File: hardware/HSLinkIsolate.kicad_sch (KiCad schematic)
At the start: 57 parts, among them J101 USB_B, J102 ISP, J103 IDC, Q101 AO3400A, SW101 BOOT, U101 HPM5301IEG1, U102 USBLC6-2SC6, U103 ISO7741, U104 ISO7741, U105 SN74LVC1G125DBV, U107 RT9193, Y101 24MHz

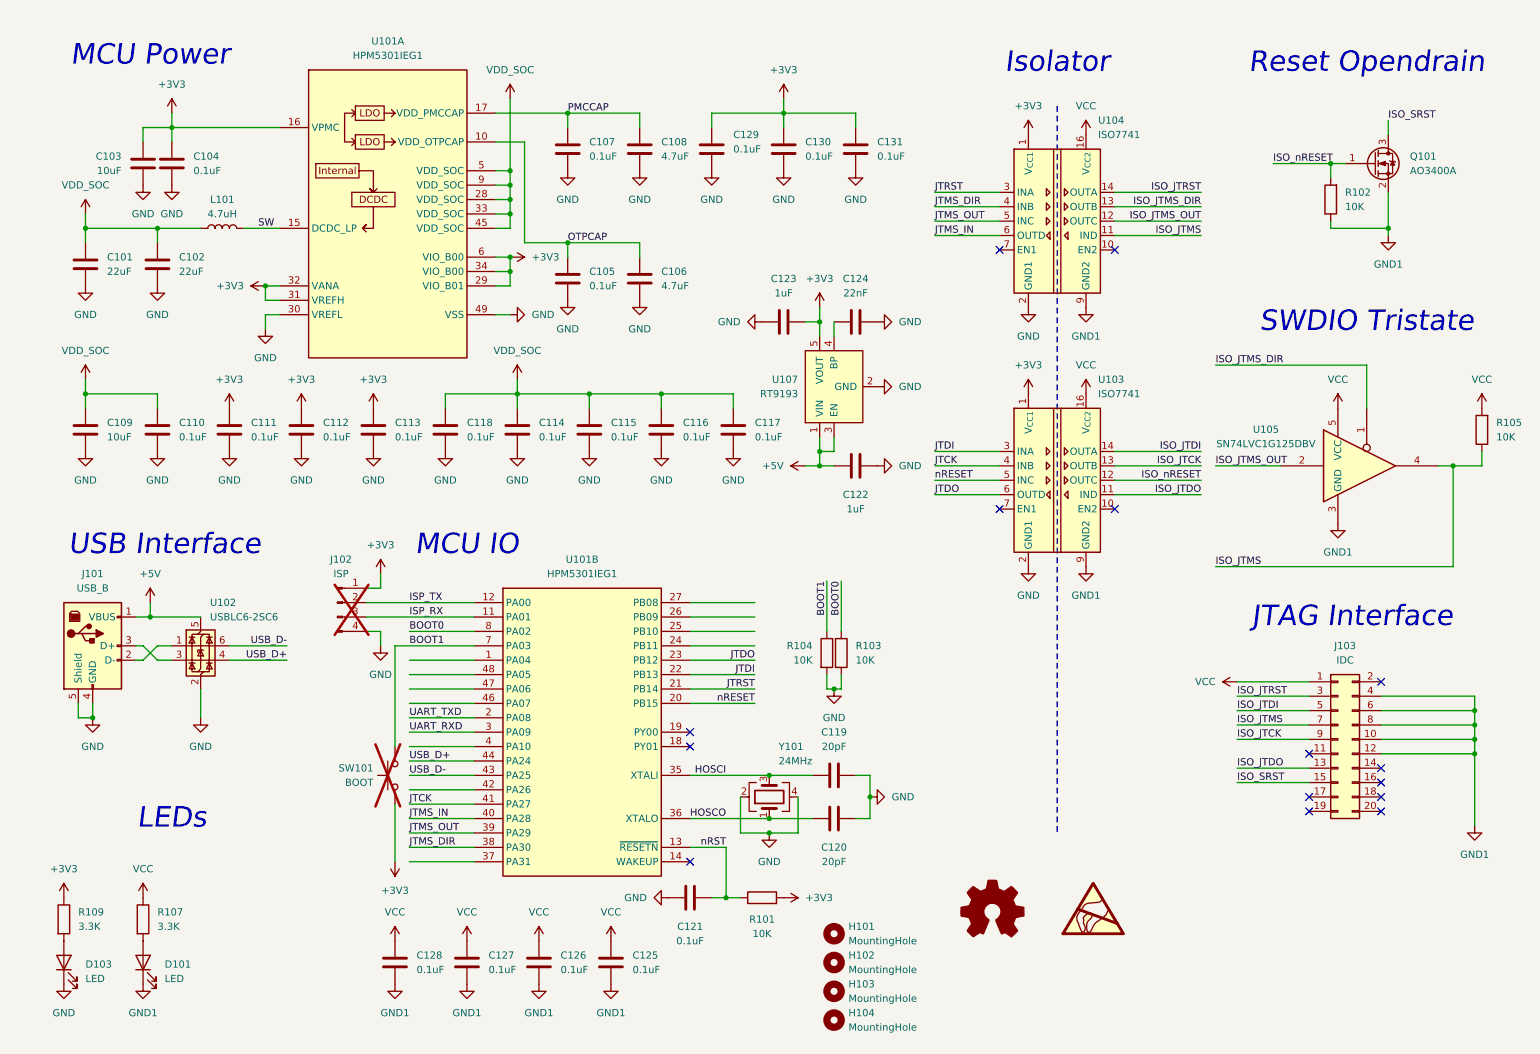
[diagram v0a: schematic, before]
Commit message: update hardware
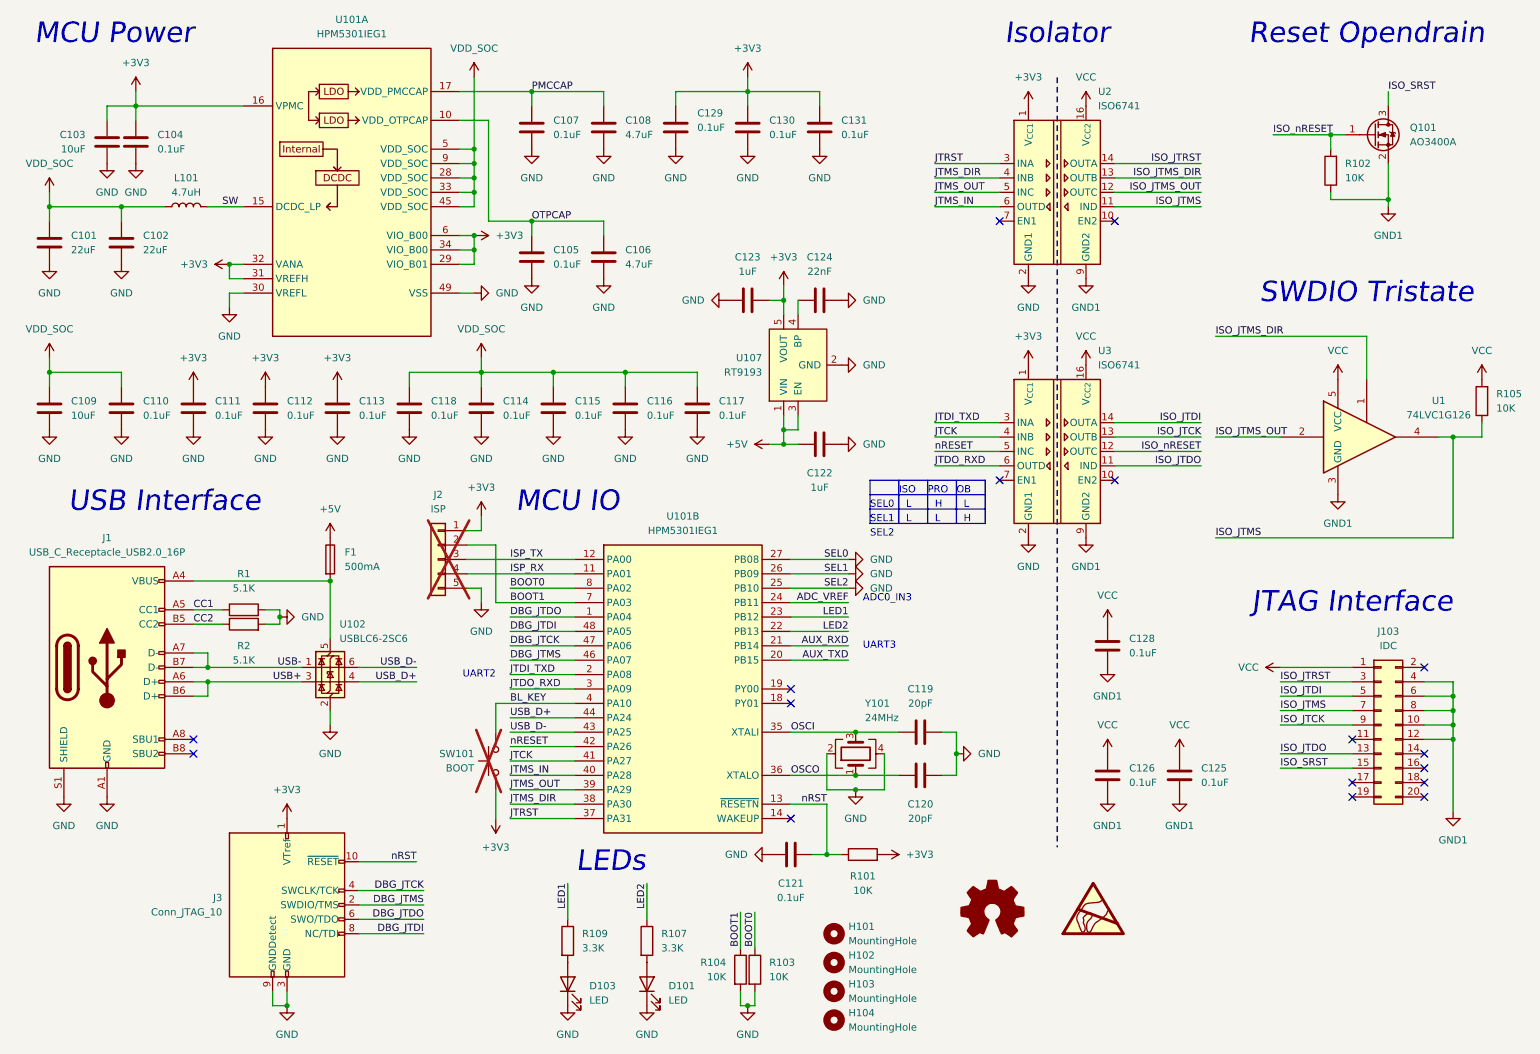
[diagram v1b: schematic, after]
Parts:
- removed C127: 0.1uF, Capacitor_SMD:C_0603_1608Metric, symbol Device:C
- removed J101: USB_B, myLib:USB_B_Lumberg_2411_02_Horizontal, symbol Connector:USB_B
- removed J102: ISP, Connector_PinHeader_2.54mm:PinHeader_1x04_P2.54mm_Vertical, symbol Connector:Conn_01x04_Pin
- removed U103, U104: ISO7741, Package_SO:QSOP-16_3.9x4.9mm_P0.635mm, symbol Isolator:ISO6741
- removed U105: SN74LVC1G125DBV, Package_TO_SOT_SMD:SOT-23-5, symbol 74xGxx:SN74LVC1G125DBV
- added F1: 500mA, Fuse:Fuse_0805_2012Metric, symbol Device:Fuse
- added J1: USB_C_Receptacle_USB2.0_16P, akaLinkIso:USB_C_Receptacle_HRO_TYPE-C-31-M-12, symbol Connector:USB_C_Receptacle_USB2.0_16P
- added J2: ISP, Connector_PinHeader_2.54mm:PinHeader_1x05_P2.54mm_Vertical, symbol Connector_Generic:Conn_01x05
- added J3: Conn_JTAG_10, Connector_PinHeader_1.27mm:PinHeader_2x05_P1.27mm_Vertical, symbol Connector:Conn_ARM_JTAG_SWD_10
- added R1, R2: 5.1K, Resistor_SMD:R_0603_1608Metric, symbol Device:R
- added U1: 74LVC1G126, Package_TO_SOT_SMD:SOT-23-5, symbol 74xGxx:74LVC1G126
- added U2, U3: ISO6741, Package_SO:SOIC-16W_7.5x10.3mm_P1.27mm, symbol Isolator:ISO6741
- H101, H102, H103, H104: footprint myLib:MountingHole_2.2mm_M2 -> akaLinkIso:MountingHole_2.5mm
- J103: footprint Connector_IDC:IDC-Header_2x10_P2.54mm_Horizontal -> akaLinkIso:IDC-Header_2x10_P2.54mm_Horizontal
- L101: footprint Inductor_SMD:L_Sunlord_SWPA4020S -> Inductor_SMD:L_Sunlord_SWPA252012S
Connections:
- net +3V3: now also J2.1 (Pin_1), J3.1 (VTref), U2.1 (V_{CC1}), U3.1 (V_{CC1}); no longer R109.1
- net +5V: now also F1.1; no longer U102.5 (VBUS)
- net BOOT1: now also J2.2 (Pin_2); no longer SW101.1
- net GND: now also D101.1 (K), U101.25 (PB10), U101.26 (PB09), U101.27 (PB08), J1.A1 (GND), J1.A12 (GND), J1.B1 (GND), J1.B12 (GND), J1.S1 (SHIELD), J2.5 (Pin_5), J3.3 (GND), J3.5 (GND), J3.9 (GNDDetect), R1.2, R2.2, U2.2 (GND1), U2.8 (GND1), U3.2 (GND1), U3.8 (GND1)
- net GND1: now also U1.3 (GND), U2.15 (GND2), U2.9 (GND2), U3.15 (GND2), U3.9 (GND2); no longer D101.1 (K)
- net ISO_JTCK: now also U3.13 (OUTB)
- net ISO_JTDI: now also U3.14 (OUTA)
- net ISO_JTDO: now also U3.11 (IND)
- net ISO_JTMS: now also U1.4, U2.11 (IND)
- net ISO_JTMS_DIR: now also U1.1, U2.13 (OUTB)
- net ISO_JTMS_OUT: now also U1.2, U2.12 (OUTC)
- net ISO_JTRST: now also U2.14 (OUTA)
- net ISO_nRESET: now also U3.12 (OUTC)
- net ISP_RX: now also J2.4 (Pin_4)
- net ISP_TX: now also J2.3 (Pin_3)
- net JTCK: now also U3.4 (INB)
- net JTMS_DIR: now also U2.4 (INB)
- net JTMS_IN: now also U2.6 (OUTD)
- net JTMS_OUT: now also U2.5 (INC)
- net JTRST: now also U101.37 (PA31), U2.3 (INA); no longer U101.21 (PB14)
- net VCC: now also U1.5 (VCC), U2.16 (V_{CC2}), U3.16 (V_{CC2}); no longer R107.1
- net nRESET: now also U101.42 (PA26), U3.5 (INC); no longer U101.20 (PB15)
- net nRST: now also J3.10 (~{RESET})
- net USB-: now reaches U102.1 (I/O1)
- net USB-: now also J1.A7 (D-), J1.B7 (D-)
- net USB+: now reaches U102.3 (I/O2)
- net USB+: now also J1.A6 (D+), J1.B6 (D+)
- net DBG_JTDO: now reaches U101.1 (PA04)
- net DBG_JTDO: now also J3.6 (SWO/TDO)
- net ADC_VREF: now reaches U101.24 (PB11)
- net BL_KEY: now reaches U101.4 (PA10)
- net BL_KEY: now also SW101.1
- net DBG_JTMS: now reaches U101.46 (PA07)
- net DBG_JTMS: now also J3.2 (SWDIO/TMS)
- net DBG_JTCK: now reaches U101.47 (PA06)
- net DBG_JTCK: now also J3.4 (SWCLK/TCK)
- net DBG_JTDI: now reaches U101.48 (PA05)
- net DBG_JTDI: now also J3.8 (NC/TDI)
- net HOSCI renamed OSCI
- net HOSCO renamed OSCO
- net JTDI renamed LED2
- net LED2: now also R107.1
- net JTDO renamed LED1
- net LED1: now also R109.1
- net UART_RXD renamed JTDO_RXD
- net JTDO_RXD: now also U3.6 (OUTD)
- net UART_TXD renamed JTDI_TXD
- net JTDI_TXD: now also U3.3 (INA)
- new net: F1.2, J1.A4 (VBUS), J1.A9 (VBUS), J1.B4 (VBUS), J1.B9 (VBUS), U102.5 (VBUS)
- new net AUX_RXD: U101.21 (PB14)
- new net AUX_TXD: U101.20 (PB15)
- new net CC1: J1.A5 (CC1), R1.1
- new net CC2: J1.B5 (CC2), R2.1
- no-connect marks 15 -> 17
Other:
- note added: "ADC0_IN3"
- note added: "H"
- note added: "ISO"
- note added: "L"
- note added: "OB"
- note added: "PRO"
- note added: "SEL0"
- note added: "SEL1"
- note added: "SEL2"
- note added: "UART2"
- note added: "UART3"
- moved on the sheet: C101, C102, C103, C104, C105, C106, C107, C108, C109, C110, C111, C112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
